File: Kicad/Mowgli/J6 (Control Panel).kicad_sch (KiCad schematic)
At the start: 29 parts, among them J6 Control Panel, Q2 NMOS_G15, Q4 NMOS_G15, Q5 NMOS_G15, Q6 NMOS_G15, SW1 CLOCK, SW3 PLAY, U2 STM32F030R8T6, U3 AMS1117-3.3

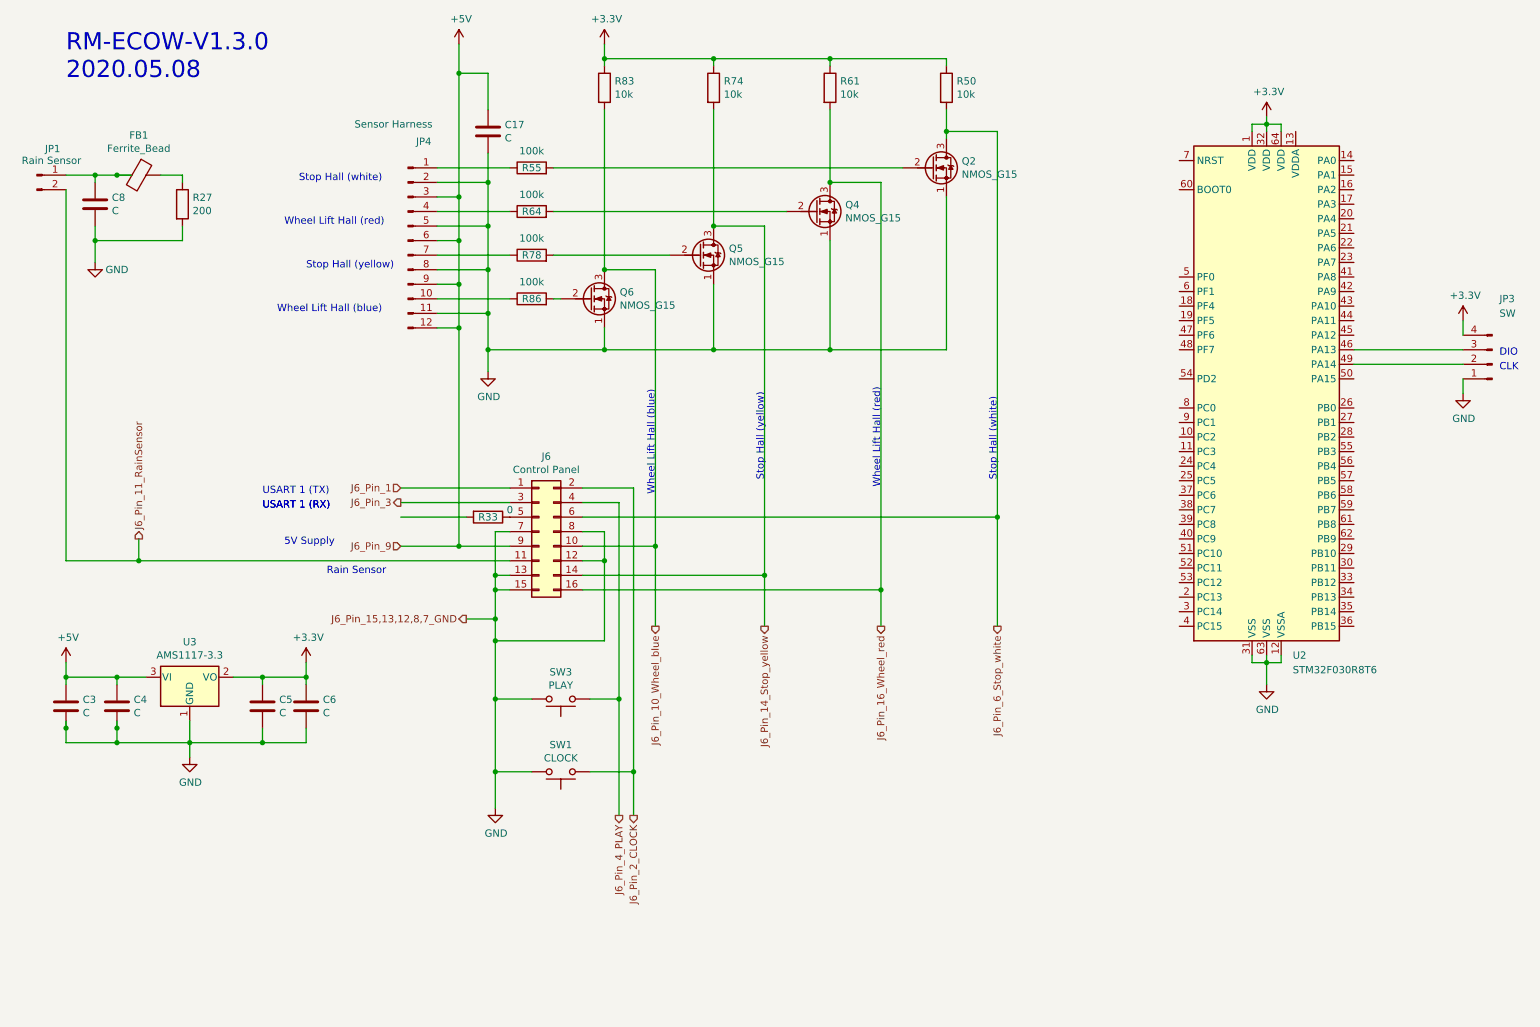
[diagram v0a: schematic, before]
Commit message: LED Labels ans some tiny stuff
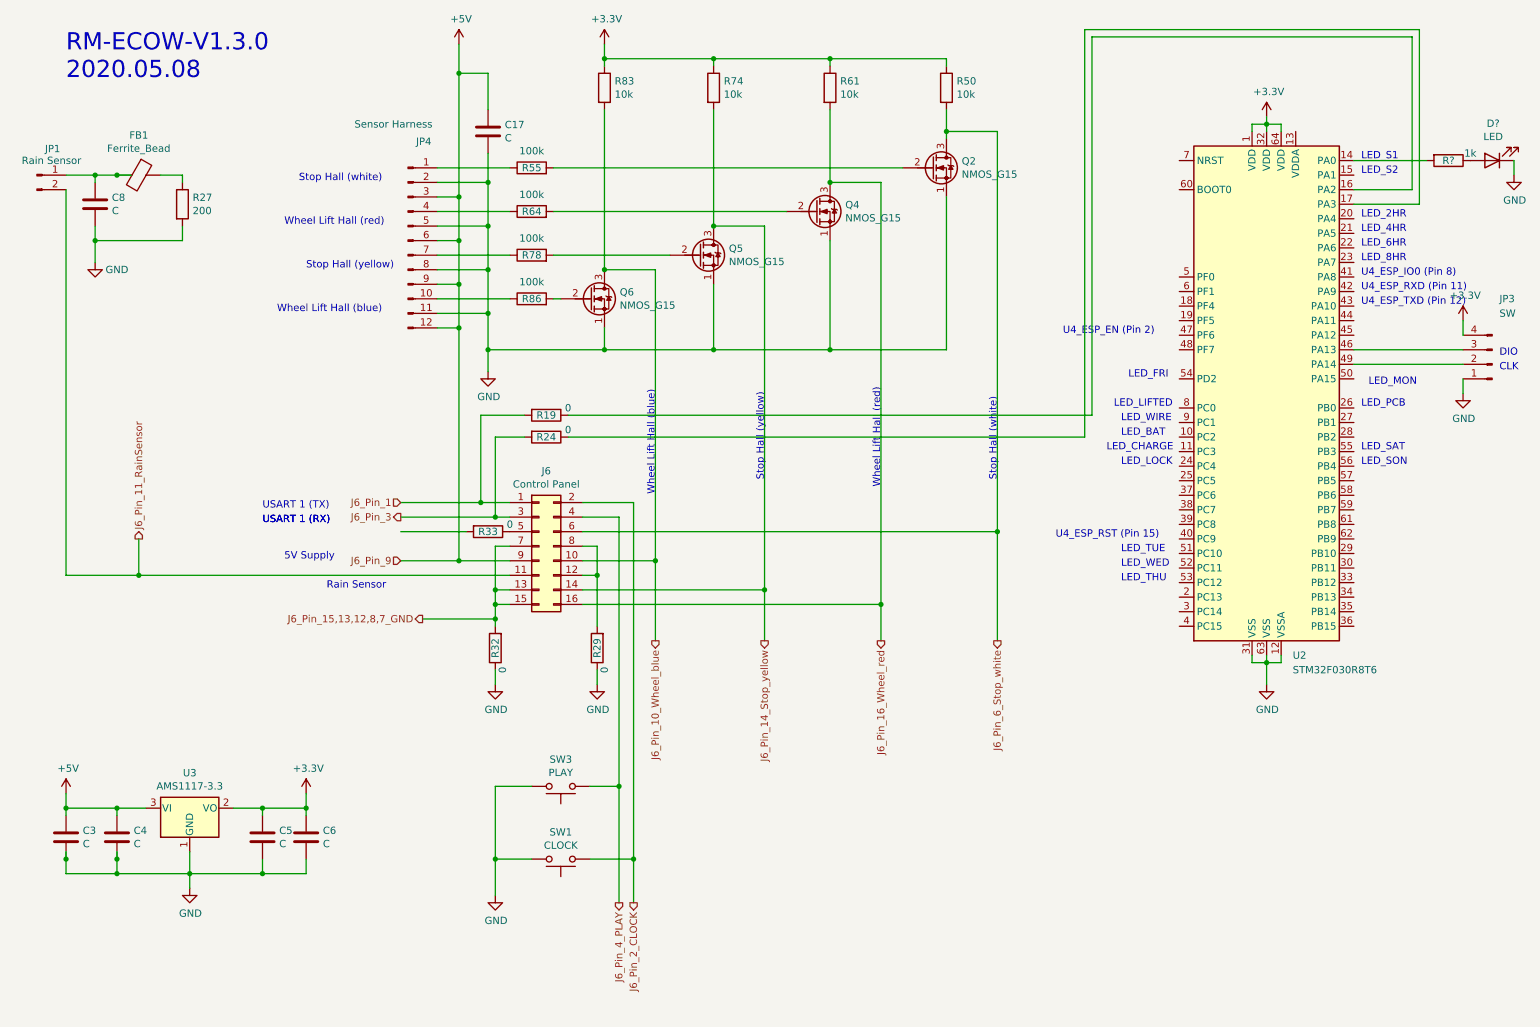
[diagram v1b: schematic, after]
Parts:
- added D?: LED, symbol Device:LED
- added R19, R24, R29, R32: 0, symbol Device:R
- added R?: 1k, symbol Device:R
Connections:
- net GND: now also D?.1 (K), R29.1, R32.1; no longer J6.12 (Pin_12), J6.13 (Pin_13), J6.15 (Pin_15), J6.7 (Pin_7), J6.8 (Pin_8)
- net J6_Pin_1: now also R19.2
- net J6_Pin_3: now also R24.2
- net at U2.14 (PA0): now also R?.2
- net at U2.16 (PA2): now also R19.1
- net at U2.17 (PA3): now also R24.1
- new net: J6.12 (Pin_12), J6.8 (Pin_8), R29.2
- new net: D?.2 (A), R?.1
- new net J6_Pin_15,13,12,8,7_GND: J6.13 (Pin_13), J6.15 (Pin_15), J6.7 (Pin_7), R32.2
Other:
- note added: "LED_2HR"
- note added: "LED_4HR"
- note added: "LED_6HR"
- note added: "LED_8HR"
- note added: "LED_BAT"
- note added: "LED_CHARGE"
- note added: "LED_FRI"
- note added: "LED_LIFTED"
- note added: "LED_LOCK"
- note added: "LED_MON"
- note added: "LED_PCB"
- note added: "LED_S1"
- note added: "LED_S2"
- note added: "LED_SAT"
- note added: "LED_SON"
- note added: "LED_THU"
- note added: "LED_TUE"
- note added: "LED_WED"
- note added: "LED_WIRE"
- note added: "U4_ESP_EN (Pin 2)"
- note added: "U4_ESP_IO0 (Pin 8)"
- note added: "U4_ESP_RST (Pin 15)"
- note added: "U4_ESP_RXD (Pin 11)"
- note added: "U4_ESP_TXD (Pin 12)"
- moved on the sheet: C3, C4, C5, C6, J6, R33, SW1, SW3, U3
